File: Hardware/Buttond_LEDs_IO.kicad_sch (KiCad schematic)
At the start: 14 parts, among them J13 SFH11-PBPC-D05-ST-BK, SW1 RESET, SW2 BOOT

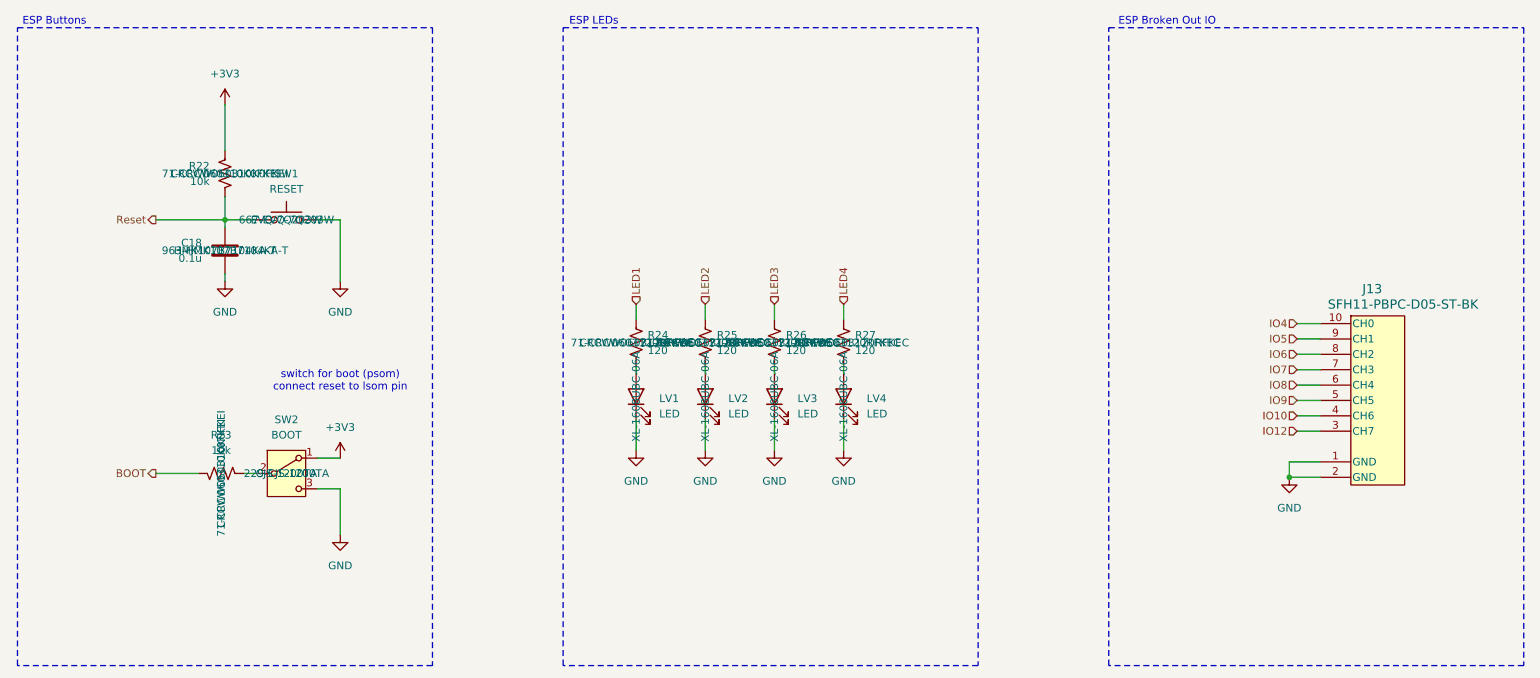
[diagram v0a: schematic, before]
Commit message: review council
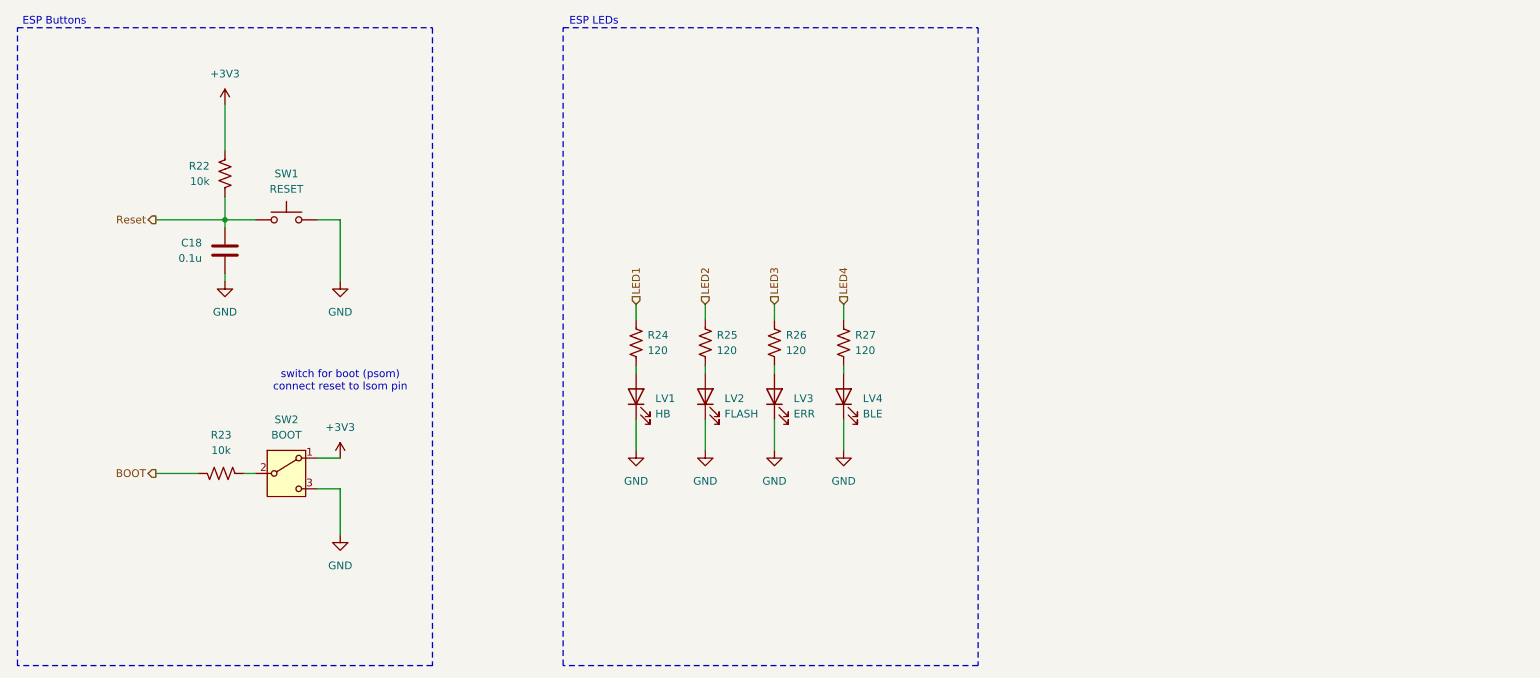
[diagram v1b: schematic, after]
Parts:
- removed J13: SFH11-PBPC-D05-ST-BK, UTSVT_Connectors:CONN_SFH11-xxxC-D05-ST-XX_SUL, symbol UTSVT_Connectors:SFH11-PBPC-D05-ST-BK
- LV1: value LED -> HB
- LV2: value LED -> FLASH
- LV3: value LED -> ERR
- LV4: value LED -> BLE
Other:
- note removed: "ESP Broken Out IO"
